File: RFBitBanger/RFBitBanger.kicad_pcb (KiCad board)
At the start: 2 copper layers, 149 x 88 mm, 236 parts, among them J1 POWER, J10 si5351mod, J11 SPEAKER, J12 Conn_Coaxial, J13 Conn_01x01, J14 Conn_01x01, J15 Conn_01x01, J16 Conn_01x01, J17 Filt1, J18 Filt2, J2 Barrel_Jack, J20 Conn_01x01, J21 Conn_01x01, J3 Conn_01x01, J4 Conn_01x01, J5 Conn_01x04, J6 Conn_01x01, J7 Conn_01x01, J8 Conn_01x01, J9 ICSP, P1 Mini-DIN_6pins_ver4, Q1 2N3904, Q10 2N3904, Q11 2N3904, Q12 2N3904, Q13 2N2907, Q14 2N3904, Q15 NC, Q2 2N3904, Q3 2N7000, Q4 2N3904, Q5 NC, Q6 2N7000, Q7 2N7000, Q8 2N2907, Q9 2N7000, SW1 SW_Push, SW2 SW_Push, SW3 SW_Push, SW4 SW_Push, SW5 SW_Push, SW6 SW_Push, T1 Trifilar, T2 Trifilar, T3 Current, T4 Common-Mode Choke, U1 ATMEGA328-PU, U2 LM7805_TO220, U3 LM386, U4 LM358, U5 LCD1602ExtraPins, U6 SI5351A, Y1 16 MHz, Y2 7.X MHz, Y3 27 MHz, Y4 7.X MHz, Y5 7.X MHz

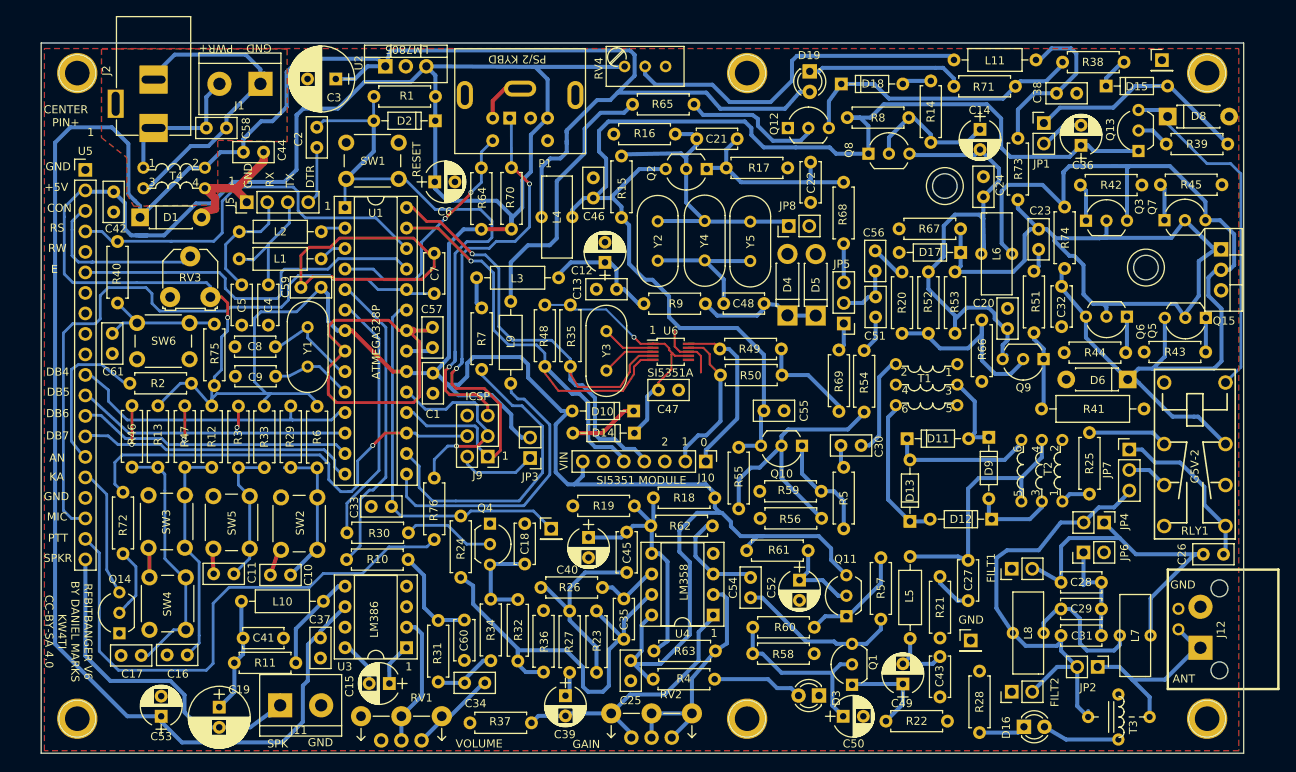
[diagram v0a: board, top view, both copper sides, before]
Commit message: Added extra row of ground pins for 40 pin connector
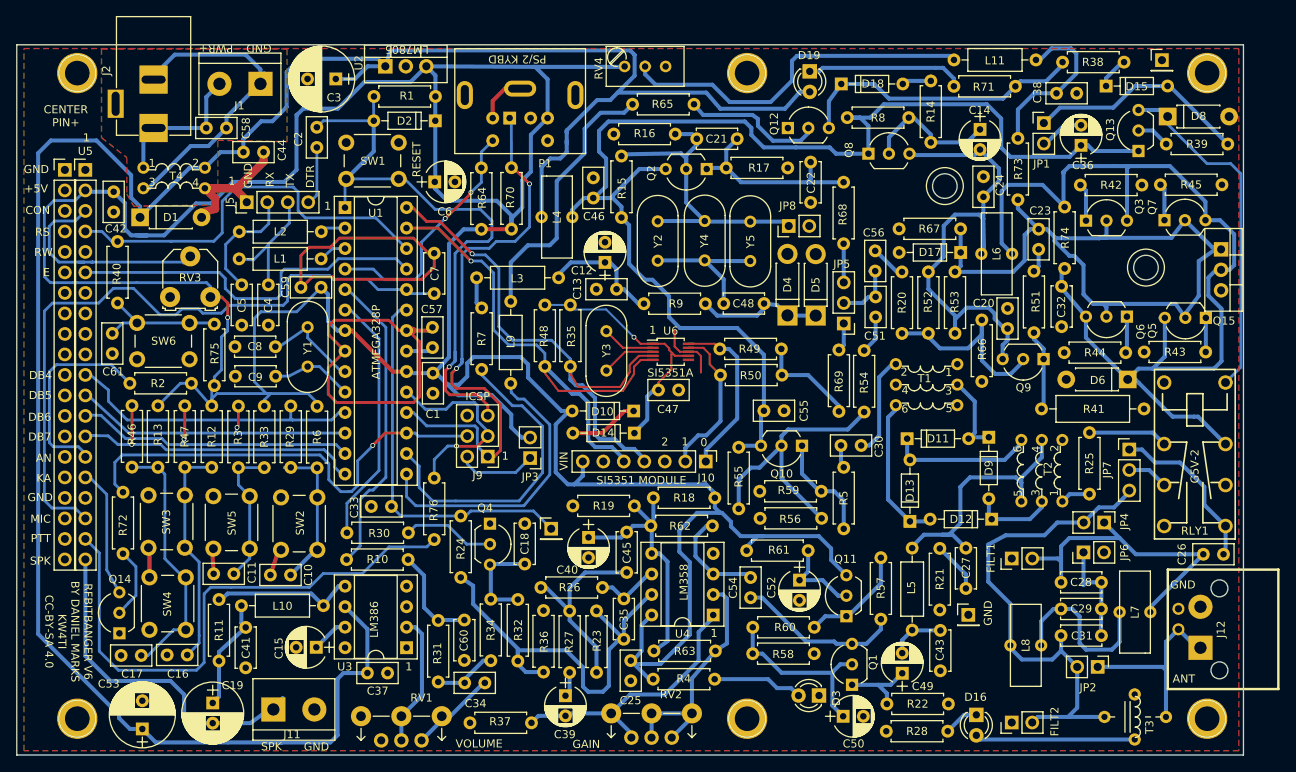
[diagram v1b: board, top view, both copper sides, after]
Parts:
- added J19: Conn_01x20, Pin_Headers:Pin_Header_Straight_1x20_Pitch2.54mm, F.Cu at (44.0, 72.5)
- C15: value NC -> 10 uF
- C53: value 100 uF -> 1000 uF; footprint Capacitors_THT:CP_Radial_D5.0mm_P2.50mm -> Capacitors_THT:CP_Radial_D8.0mm_P3.50mm
- moved R28 13.8 mm to (145.7, 142.1), turned to 0 degrees
- moved C15 10.1 mm to (75.1, 131.7)
- moved C37 7.27 mm to (81.5, 134.8), turned to 0 degrees
- moved D16 6.08 mm to (156.9, 140.0), turned to 270 degrees
- moved J18 3.81 mm to (161.3, 141.0)
- moved R21 3.48 mm to (152.4, 127.0)
- moved C43 3.24 mm to (152.4, 129.6)
- moved J15 3.19 mm to (155.9, 127.6)
- moved L7 2.90 mm to (176.6, 127.3)
- moved C53 2.82 mm to (53.6, 141.8)
- moved R22 2.13 mm to (145.8, 138.7)
- moved T3 2.03 mm to (176.6, 140.3)
- moved R11 1.91 mm to (63.1, 133.3), turned to 90 degrees
- moved L8 1.56 mm to (163.0, 131.4)
- moved C27 1.53 mm to (155.6, 124.4)
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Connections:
- C15 pad 2: Net-(C15-Pad2) -> GND
- U3 pad 1: Net-(C15-Pad1) -> (no net)
- U3 pad 7: (no net) -> Net-(C15-Pad1)
- U3 pad 8: Net-(C15-Pad2) -> (no net)
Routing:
- net Net-(D16-Pad2): track 9.59 -> 19.8 mm
- net Net-(C31-Pad2): track 57.7 -> 63.8 mm
- net Net-(C15-Pad2): track 5.95 -> 0.00 mm
- net Net-(RV3-Pad2): track 24.2 -> 30.1 mm
- net Net-(R2-Pad1): track 21.2 -> 27.0 mm
- net +12V: track 273.4 -> 279.1 mm
- net Net-(L10-Pad1): track 13.0 -> 18.3 mm
- net +5V: track 416.4 -> 421.3 mm
- net MICPADDLE: track 82.7 -> 87.6 mm
- net Net-(C29-Pad2): track 17.9 -> 22.3 mm
- net Net-(C26-Pad2): track 43.9 -> 40.7 mm
- net Net-(C49-Pad1): track 12.1 -> 9.77 mm
- net Net-(C43-Pad1): track 8.91 -> 6.87 mm
- net Net-(C19-Pad1): track 15.1 -> 16.8 mm
- net Net-(D16-Pad1): track 5.80 -> 4.38 mm
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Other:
- board size 149 x 88 mm -> 152 x 88 mm
- board text removed: "SPKR"
